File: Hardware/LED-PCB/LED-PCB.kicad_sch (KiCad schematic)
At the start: 225 parts, among them J1 Conn_01x03_Pin

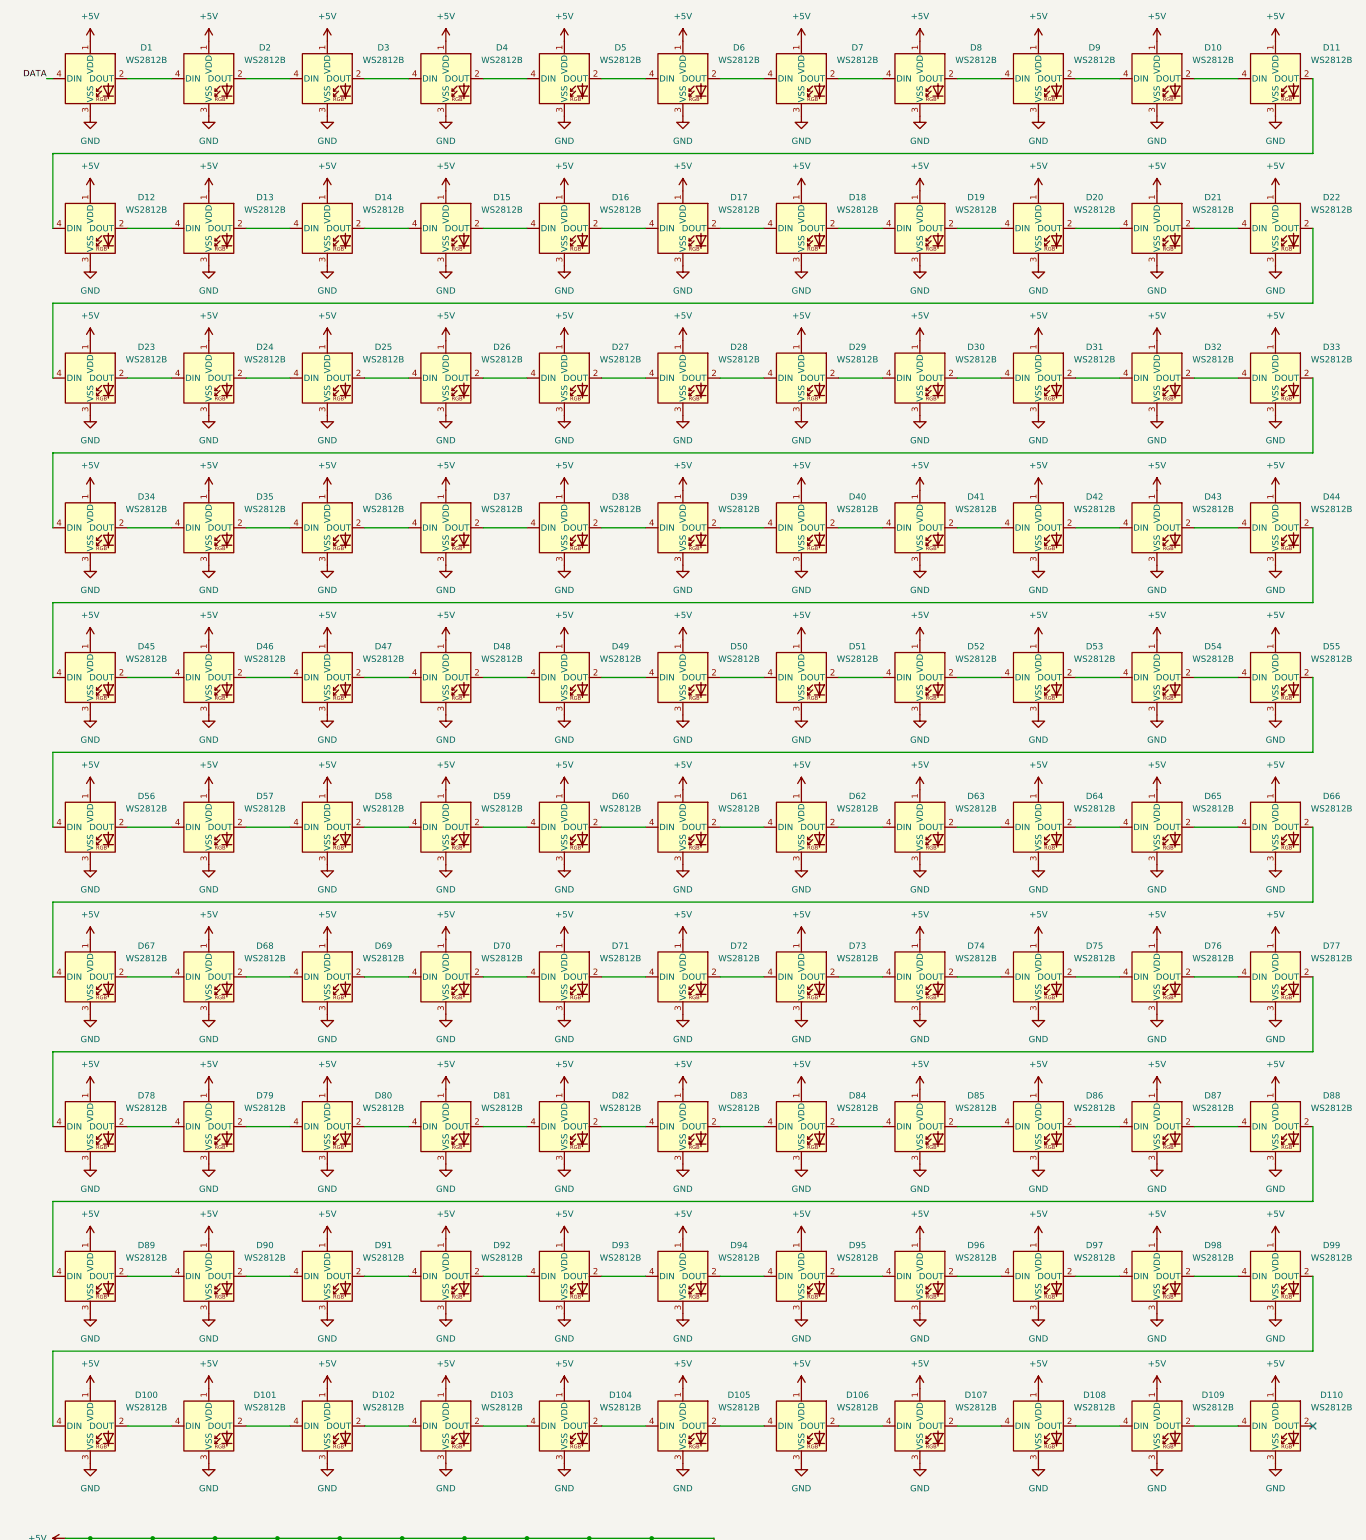
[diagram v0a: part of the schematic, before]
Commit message: led placed
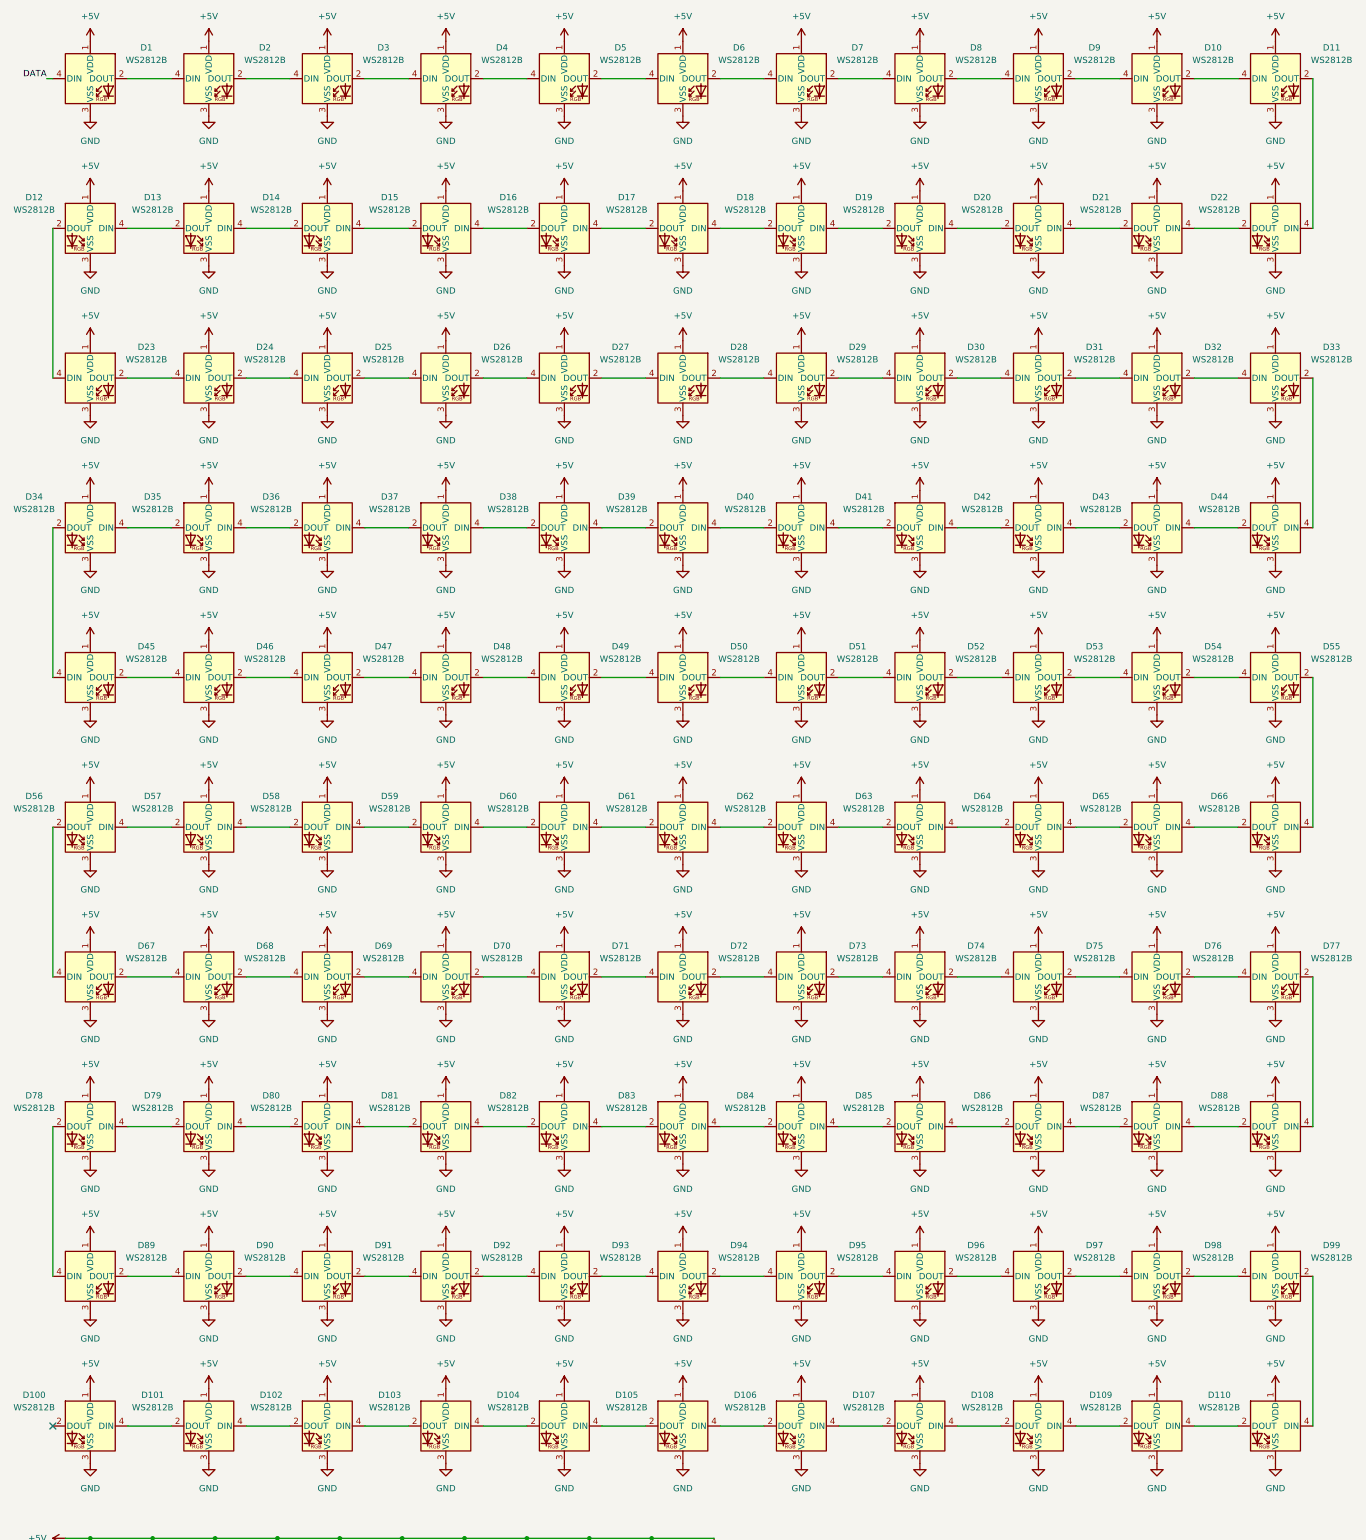
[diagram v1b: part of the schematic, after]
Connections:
- net at D14.2 (DOUT): now also D13.4 (DIN); no longer D15.4 (DIN)
- net at D14.4 (DIN): now also D15.2 (DOUT); no longer D13.2 (DOUT)
- net at D81.2 (DOUT): now also D80.4 (DIN); no longer D82.4 (DIN)
- net at D81.4 (DIN): now also D82.2 (DOUT); no longer D80.2 (DOUT)
- net at D41.2 (DOUT): now also D40.4 (DIN); no longer D42.4 (DIN)
- net at D41.4 (DIN): now also D42.2 (DOUT); no longer D40.2 (DOUT)
- net at D63.2 (DOUT): now also D62.4 (DIN); no longer D64.4 (DIN)
- net at D63.4 (DIN): now also D64.2 (DOUT); no longer D62.2 (DOUT)
- net at D23.4 (DIN): now also D12.2 (DOUT); no longer D22.2 (DOUT)
- net at D12.4 (DIN): now also D13.2 (DOUT); no longer D11.2 (DOUT)
- net at D34.2 (DOUT): now also D45.4 (DIN); no longer D35.4 (DIN)
- net at D34.4 (DIN): now also D35.2 (DOUT); no longer D33.2 (DOUT)
- net at D79.2 (DOUT): now also D78.4 (DIN); no longer D80.4 (DIN)
- net at D79.4 (DIN): now also D80.2 (DOUT); no longer D78.2 (DOUT)
- net at D87.2 (DOUT): now also D86.4 (DIN); no longer D88.4 (DIN)
- net at D87.4 (DIN): now also D88.2 (DOUT); no longer D86.2 (DOUT)
- net at D107.2 (DOUT): now also D106.4 (DIN); no longer D108.4 (DIN)
- net at D107.4 (DIN): now also D108.2 (DOUT); no longer D106.2 (DOUT)
- net at D36.2 (DOUT): now also D35.4 (DIN); no longer D37.4 (DIN)
- net at D36.4 (DIN): now also D37.2 (DOUT); no longer D35.2 (DOUT)
- net at D102.2 (DOUT): now also D101.4 (DIN); no longer D103.4 (DIN)
- net at D102.4 (DIN): now also D103.2 (DOUT); no longer D101.2 (DOUT)
- net at D100.2 (DOUT): no longer D101.4 (DIN)
- net at D16.2 (DOUT): now also D15.4 (DIN); no longer D17.4 (DIN)
- net at D16.4 (DIN): now also D17.2 (DOUT); no longer D15.2 (DOUT)
- net at D22.4 (DIN): now also D11.2 (DOUT); no longer D21.2 (DOUT)
- net at D58.2 (DOUT): now also D57.4 (DIN); no longer D59.4 (DIN)
- net at D58.4 (DIN): now also D59.2 (DOUT); no longer D57.2 (DOUT)
- net at D38.4 (DIN): now also D39.2 (DOUT); no longer D37.2 (DOUT)
- net at D100.4 (DIN): now also D101.2 (DOUT); no longer D99.2 (DOUT)
- net at D61.2 (DOUT): now also D60.4 (DIN); no longer D62.4 (DIN)
- net at D61.4 (DIN): now also D62.2 (DOUT); no longer D60.2 (DOUT)
- net at D43.2 (DOUT): now also D42.4 (DIN); no longer D44.4 (DIN)
- net at D43.4 (DIN): now also D44.2 (DOUT); no longer D42.2 (DOUT)
- net at D77.2 (DOUT): now also D88.4 (DIN); no longer D78.4 (DIN)
- net at D109.4 (DIN): now also D110.2 (DOUT); no longer D108.2 (DOUT)
- net at D104.4 (DIN): now also D105.2 (DOUT); no longer D103.2 (DOUT)
- net at D89.4 (DIN): now also D78.2 (DOUT); no longer D88.2 (DOUT)
- net at D56.2 (DOUT): now also D67.4 (DIN); no longer D57.4 (DIN)
- net at D66.2 (DOUT): now also D65.4 (DIN); no longer D67.4 (DIN)
- net at D66.4 (DIN): now also D55.2 (DOUT); no longer D65.2 (DOUT)
- net at D18.4 (DIN): now also D19.2 (DOUT); no longer D17.2 (DOUT)
- net at D38.2 (DOUT): now also D37.4 (DIN); no longer D39.4 (DIN)
- net at D104.2 (DOUT): now also D103.4 (DIN); no longer D105.4 (DIN)
- net at D18.2 (DOUT): now also D17.4 (DIN); no longer D19.4 (DIN)
- net at D56.4 (DIN): now also D57.2 (DOUT); no longer D55.2 (DOUT)
- net at D20.4 (DIN): now also D21.2 (DOUT); no longer D19.2 (DOUT)
- net at D110.4 (DIN): now also D99.2 (DOUT); no longer D109.2 (DOUT)
- net at D21.4 (DIN): now also D22.2 (DOUT); no longer D20.2 (DOUT)
- net at D83.2 (DOUT): now also D82.4 (DIN); no longer D84.4 (DIN)
- net at D83.4 (DIN): now also D84.2 (DOUT); no longer D82.2 (DOUT)
- net at D85.2 (DOUT): now also D84.4 (DIN); no longer D86.4 (DIN)
- net at D85.4 (DIN): now also D86.2 (DOUT); no longer D84.2 (DOUT)
- new net: D108.4 (DIN), D109.2 (DOUT)
- new net: D33.2 (DOUT), D44.4 (DIN)
- new net: D59.4 (DIN), D60.2 (DOUT)
- new net: D19.4 (DIN), D20.2 (DOUT)
- new net: D105.4 (DIN), D106.2 (DOUT)
- new net: D39.4 (DIN), D40.2 (DOUT)
- new net: D64.4 (DIN), D65.2 (DOUT)
